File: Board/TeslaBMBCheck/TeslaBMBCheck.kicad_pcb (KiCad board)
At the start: 2 copper layers, 99.4 x 60.2 mm, 35 parts, among them J1 TESLA_BMS, J9 ICSP, Q1 IRLML2244, Q2 BSS138, U1 USBLC6, U2 PIC18F2480-ISO, Y1 10 MHz

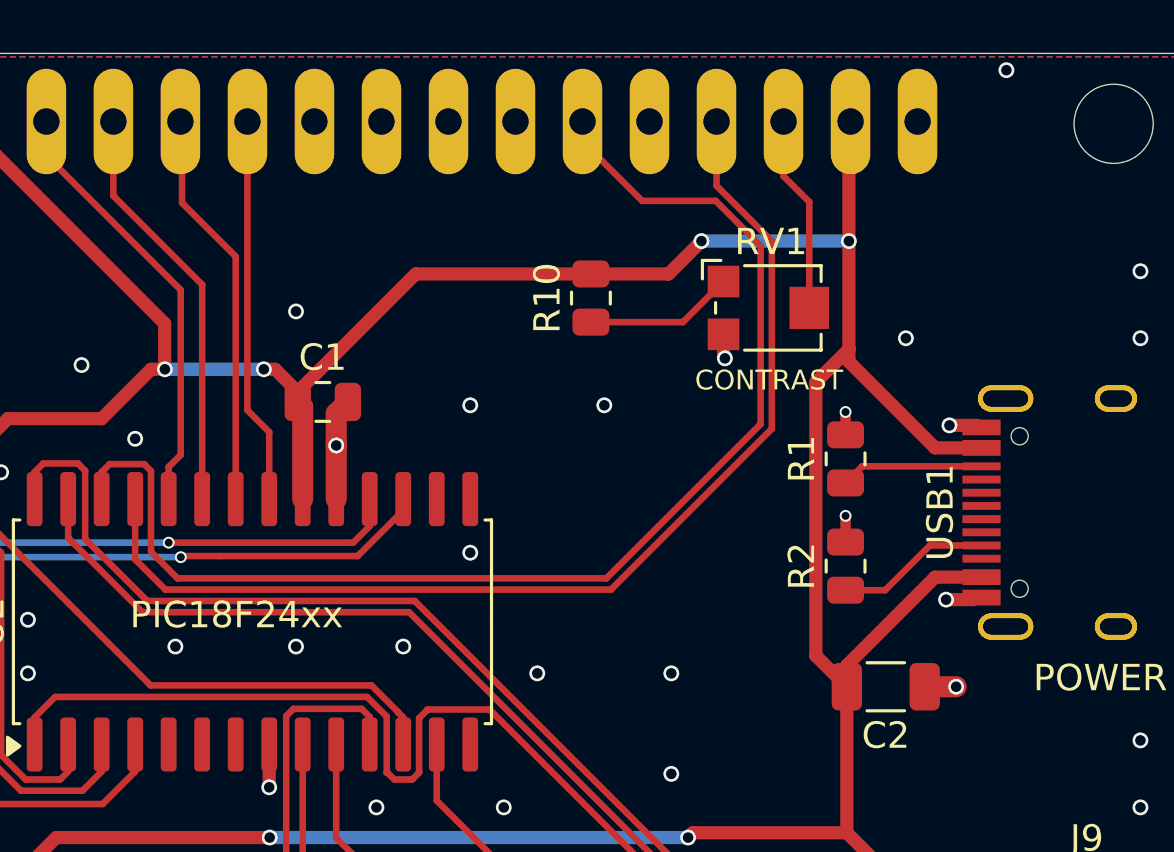
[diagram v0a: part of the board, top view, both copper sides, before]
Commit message: Minor improvements
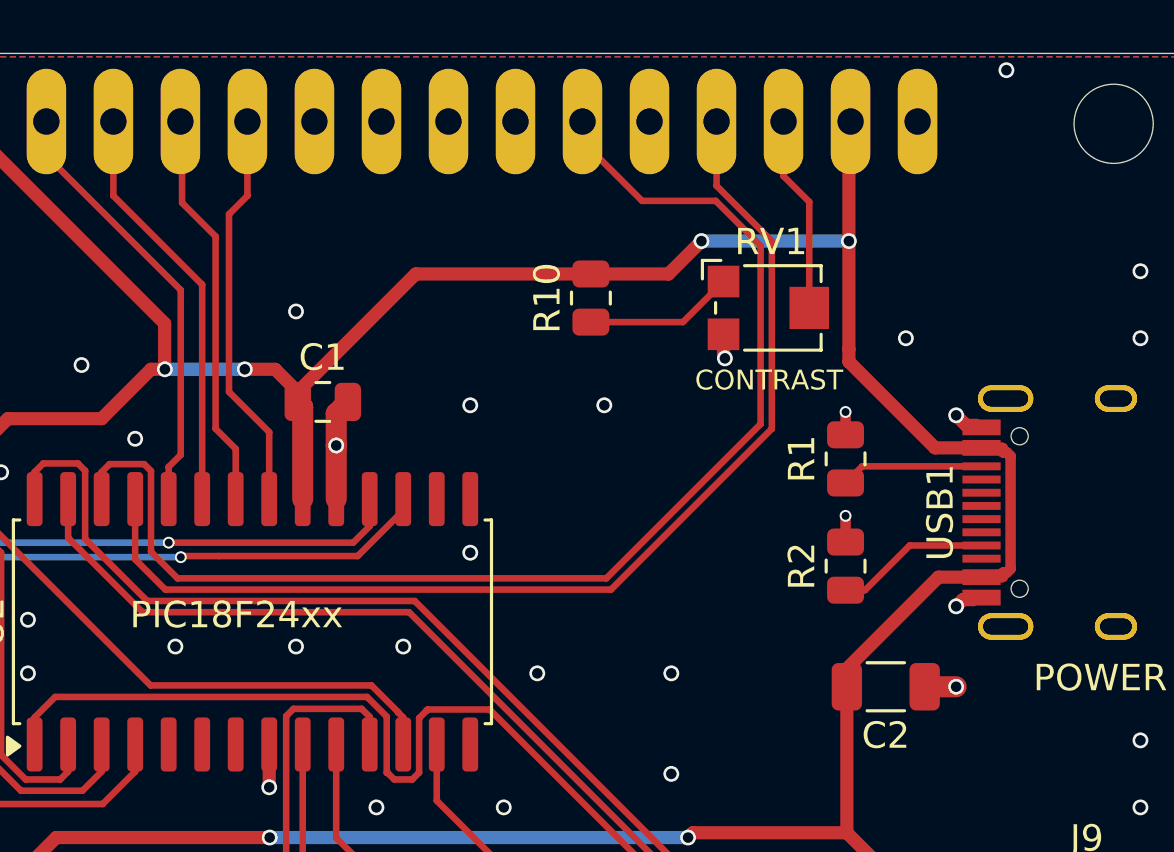
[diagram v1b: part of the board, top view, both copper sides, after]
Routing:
- net VCC: track 200.5 -> 192.9 mm
- net /LCD_D4: track 14.7 -> 15.2 mm
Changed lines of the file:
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@@
+	)
+	(segment
+		(start 166.497 61.722)
+		(end 166.574 61.799)
+		(width 0.5)
+		(layer "F.Cu")
+		(net 1)
 	)
 	(segment
@@
 	)
 	(segment
-		(start 165.481 61.722)
-		(end 166.497 61.722)
-		(width 0.5)
-		(layer "F.Cu")
-		(net 1)
-	)
-	(segment
 		(start 80.772 62.992)
 		(end 80.772 61.722)
@@
 	)
 	(segment
-		(start 166.37 68.326)
-		(end 166.447 68.249)
-		(width 0.5)
-		(layer "F.Cu")
-		(net 1)
-	)
-	(segment
-		(start 165.354 68.326)
-		(end 166.37 68.326)
+		(start 166.447 68.249)
+		(end 166.697 68.249)
 		(width 0.5)
 		(layer "F.Cu")
@@
 	)
 	(segment
+		(start 166.37 68.326)
+		(end 166.447 68.249)
+		(width 0.5)
+		(layer "F.Cu")
+		(net 1)
+	)
+	(segment
 		(start 114.5032 102.6622)
 		(end 114.5032 103.7082)
 		(width 0.25)
+		(layer "F.Cu")
+		(net 1)
+	)
+	(segment
+		(start 165.735 61.341)
+		(end 166.116 61.722)
+		(width 0.5)
 		(layer "F.Cu")
 		(net 1)
@@
 	)
 	(segment
-		(start 166.447 68.249)
-		(end 166.697 68.249)
-		(width 0.5)
-		(layer "F.Cu")
-		(net 1)
-	)
-	(segment
 		(start 80.772 79.248)
 		(end 80.772 77.978)
@@
 	)
 	(segment
+		(start 165.989 68.326)
+		(end 166.37 68.326)
+		(width 0.5)
+		(layer "F.Cu")
+		(net 1)
+	)
+	(segment
 		(start 139.378 87.884)
 		(end 140.462 87.884)
@@
 	)
 	(segment
+		(start 166.116 61.722)
+		(end 166.497 61.722)
+		(width 0.5)
+		(layer "F.Cu")
+		(net 1)
+	)
+	(segment
 		(start 83.693 100.203)
 		(end 83.693 99.06)
@@
 	)
 	(segment
-		(start 166.497 61.722)
-		(end 166.574 61.799)
+		(start 165.735 68.58)
+		(end 165.989 68.326)
 		(width 0.5)
 		(layer "F.Cu")
@@
 	)
 	(via
-		(at 165.481 61.722)
+		(at 165.735 61.341)
 		(size 0.6)
 		(drill 0.4)
@@
 	)
 	(via
-		(at 165.354 68.326)
+		(at 165.735 68.58)
 		(size 0.6)
 		(drill 0.4)
@@
 	)
 	(segment
+		(start 166.697 62.574)
+		(end 167.48457 62.574)
+		(width 0.4)
+		(layer "F.Cu")
+		(net 2)
+	)
+	(segment
+		(start 167.65857 62.748)
+		(end 167.798 62.88743)
+		(width 0.4)
+		(layer "F.Cu")
+		(net 2)
+	)
+	(segment
 		(start 140.97 61.021)
 		(end 140.782 60.833)
@@
 	)
 	(segment
+		(start 167.513 62.748)
+		(end 167.65857 62.748)
+		(width 0.4)
+		(layer "F.Cu")
+		(net 2)
+	)
+	(segment
 		(start 170.688 82.296)
 		(end 170.0276 81.6356)
@@
 	)
 	(segment
-		(start 160.418 60.085654)
-		(end 160.418 70.453)
-		(width 0.5)
-		(layer "F.Cu")
-		(net 2)
-	)
-	(segment
 		(start 155.7565 77.1615)
 		(end 155.575 77.343)
@@
 	)
 	(segment
-		(start 164.936 67.474)
-		(end 161.593 70.817)
-		(width 0.5)
+		(start 167.513 62.60243)
+		(end 167.513 62.748)
+		(width 0.4)
 		(layer "F.Cu")
 		(net 2)
@@
 	)
 	(segment
+		(start 167.48457 62.574)
+		(end 167.513 62.60243)
+		(width 0.4)
+		(layer "F.Cu")
+		(net 2)
+	)
+	(segment
 		(start 123.341 66.5261)
 		(end 123.4899 66.675)
@@
 	)
 	(segment
-		(start 139.4968 59.596)
-		(end 139.926 59.596)
-		(width 0.5)
-		(layer "F.Cu")
-		(net 2)
-	)
-	(segment
 		(start 97.660004 64.23245)
 		(end 124.43045 64.23245)
@@
 	)
 	(segment
-		(start 166.697 67.474)
-		(end 164.936 67.474)
-		(width 0.5)
-		(layer "F.Cu")
-		(net 2)
-	)
-	(segment
 		(start 145.2505 55.9835)
 		(end 140.782 60.452)
@@
 	)
 	(segment
-		(start 161.593 71.325)
-		(end 161.593 71.628)
+		(start 167.48457 67.474)
+		(end 166.697 67.474)
 		(width 0.4)
 		(layer "F.Cu")
@@
 	)
 	(segment
+		(start 161.593 70.944)
+		(end 161.593 71.628)
+		(width 0.5)
+		(layer "F.Cu")
+		(net 2)
+	)
+	(segment
 		(start 128.0945 80.8755)
 		(end 131.627 77.343)
@@
 		(end 127.9652 63.2968)
 		(width 0.5)
+		(layer "F.Cu")
+		(net 2)
+	)
+	(segment
+		(start 167.513 67.3)
+		(end 167.513 67.44557)
+		(width 0.4)
+		(layer "F.Cu")
+		(net 2)
+	)
+	(segment
+		(start 167.798 67.16057)
+		(end 167.65857 67.3)
+		(width 0.4)
 		(layer "F.Cu")
 		(net 2)
@@
 	)
 	(segment
+		(start 167.798 62.88743)
+		(end 167.798 67.16057)
+		(width 0.4)
+		(layer "F.Cu")
+		(net 2)
+	)
+	(segment
 		(start 166.116 81.6845)
 		(end 161.593 77.1615)
@@
 	)
 	(segment
-		(start 161.593 70.817)
-		(end 161.593 71.628)
-		(width 0.5)
-		(layer "F.Cu")
-		(net 2)
-	)
-	(segment
-		(start 161.593 71.328702)
-		(end 161.593 71.628)
-		(width 0.4)
+		(start 165.063 67.474)
+		(end 161.593 70.944)
+		(width 0.5)
+		(layer "F.Cu")
+		(net 2)
+	)
+	(segment
+		(start 166.697 67.474)
+		(end 165.063 67.474)
+		(width 0.5)
+		(layer "F.Cu")
+		(net 2)
+	)
+	(segment
+		(start 139.926 59.596)
+		(end 140.782 60.452)
+		(width 0.5)
+		(layer "F.Cu")
+		(net 2)
+	)
+	(segment
+		(start 138.776 59.596)
+		(end 139.926 59.596)
+		(width 0.5)
 		(layer "F.Cu")
 		(net 2)
@@
 	)
 	(segment
-		(start 161.671 58.832654)
-		(end 160.418 60.085654)
-		(width 0.5)
-		(layer "F.Cu")
-		(net 2)
-	)
-	(segment
-		(start 139.926 59.596)
-		(end 140.782 60.452)
-		(width 0.5)
+		(start 167.513 67.44557)
+		(end 167.48457 67.474)
+		(width 0.4)
 		(layer "F.Cu")
 		(net 2)
@@
 	)
 	(segment
+		(start 167.65857 67.3)
+		(end 167.513 67.3)
+		(width 0.4)
+		(layer "F.Cu")
+		(net 2)
+	)
+	(segment
 		(start 161.671 59.309)
 		(end 161.671 58.832654)
@@
 	)
 	(segment
-		(start 160.418 70.453)
-		(end 161.593 71.628)
-		(width 0.5)
-		(layer "F.Cu")
-		(net 2)
-	)
-	(segment
 		(start 154.8365 55.9835)
 		(end 156.083 54.737)
@@
 	)
 	(via
-		(at 139.4968 59.596)
+		(at 138.776 59.596)
 		(size 0.6)
 		(drill 0.4)
@@
 	)
 	(segment
-		(start 135.7472 59.596)
-		(end 139.4968 59.596)
-		(width 0.5)
-		(layer "B.Cu")
-		(net 2)
-	)
-	(segment
 		(start 124.43045 64.23245)
 		(end 125.2137 63.4492)
@@
 	)
 	(segment
+		(start 135.7472 59.596)
+		(end 138.776 59.596)
+		(width 0.5)
+		(layer "B.Cu")
+		(net 2)
+	)
+	(segment
 		(start 156.083 54.737)
 		(end 161.671 54.737)
@@
 	)
 	(segment
-		(start 138.8738 61.1498)
+		(start 138.8738 53.0232)
 		(end 138.8738 50.20586)
 		(width 0.25)
@@
 	)
 	(segment
+		(start 138.176 53.721)
+		(end 138.8738 53.0232)
+		(width 0.25)
+		(layer "F.Cu")
+		(net 8)
+	)
+	(segment
+		(start 138.176 60.452)
+		(end 138.176 53.721)
+		(width 0.25)
+		(layer "F.Cu")
+		(net 8)
+	)
+	(segment
 		(start 139.7 61.976)
-		(end 138.8738 61.1498)
+		(end 138.176 60.452)
 		(width 0.25)
 		(layer "F.Cu")
@@
 	)
 	(segment
-		(start 138.43 55.3212)
-		(end 136.398 53.2892)
+		(start 137.668 61.849)
+		(end 137.668 54.5592)
+		(width 0.25)
+		(layer "F.Cu")
+		(net 15)
+	)
+	(segment
+		(start 138.43 62.611)
+		(end 137.668 61.849)
+		(width 0.25)
+		(layer "F.Cu")
+		(net 15)
+	)
+	(segment
+		(start 138.43 64.516)
+		(end 138.43 62.611)
 		(width 0.25)
 		(layer "F.Cu")
@@
 	)
 	(segment
-		(start 138.43 64.516)
-		(end 138.43 55.3212)
-		(width 0.25)
-		(layer "F.Cu")
-		(net 15)
-	)
-	(segment
 		(start 136.398 53.2892)
 		(end 136.398 50.27006)
@@
 	)
 	(segment
+		(start 137.668 54.5592)
+		(end 136.398 53.2892)
+		(width 0.25)
+		(layer "F.Cu")
+		(net 15)
+	)
+	(segment
 		(start 99.65 100.23)
 		(end 99.65 87.199546)
@@
 	)
 	(segment
-		(start 163.0445 67.9685)
+		(start 162.2825 67.9685)
 		(end 161.544 67.9685)
 		(width 0.25)
@@
 	)
 	(segment
-		(start 164.739 66.274)
-		(end 163.0445 67.9685)
+		(start 163.977 66.274)
+		(end 162.2825 67.9685)
 		(width 0.25)
 		(layer "F.Cu")
@@
 	(segment
 		(start 166.697 66.274)
-		(end 164.739 66.274)
-		(width 0.25)
-		(layer "F.Cu")
+		(end 163.977 66.274)
+		(width 0.25)
+		(layer "F.Cu")
